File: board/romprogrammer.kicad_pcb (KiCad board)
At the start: 2 copper layers, 5 parts, among them U1 ARDUINO_NANO_V3, U2 74HC595, U3 74HC595, U4 74HC595, U5 SST39SF020

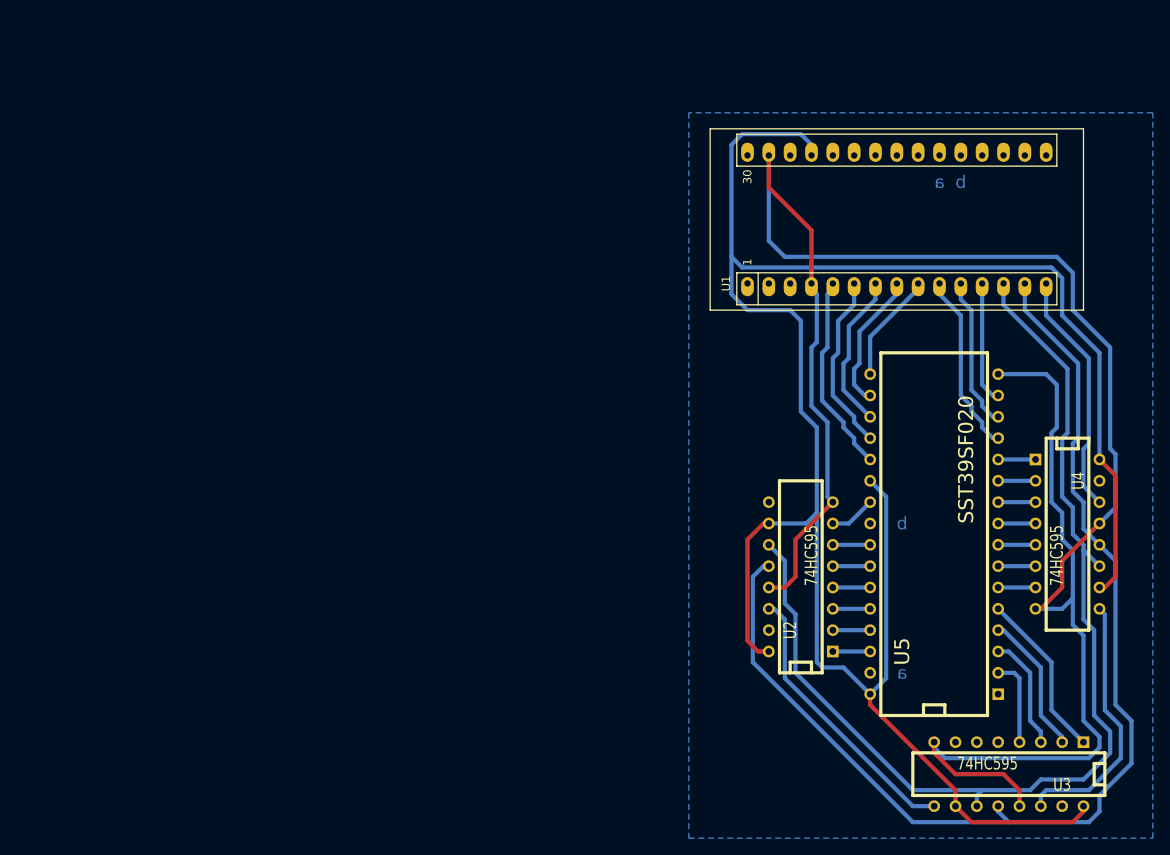
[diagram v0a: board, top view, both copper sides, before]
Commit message: fo
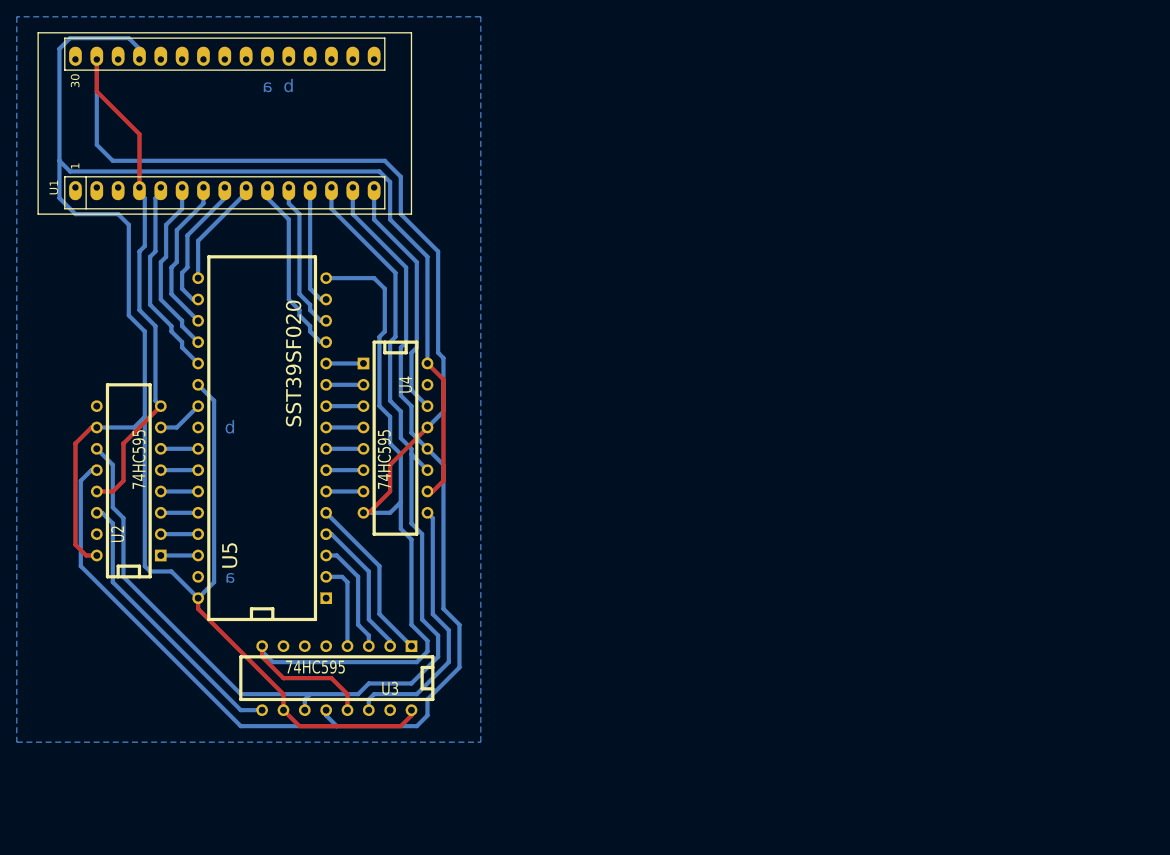
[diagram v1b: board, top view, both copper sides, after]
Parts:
- moved U1 80.8 mm to (52.7, 33.7)
- moved U2 80.8 mm to (41.9, 76.8)
- moved U3 80.8 mm to (66.7, 100.3)
- moved U4 80.8 mm to (73.7, 71.8)
- moved U5 80.8 mm to (57.8, 71.8)
